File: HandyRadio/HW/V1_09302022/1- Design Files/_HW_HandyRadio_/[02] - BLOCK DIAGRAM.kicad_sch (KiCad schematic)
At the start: 0 parts

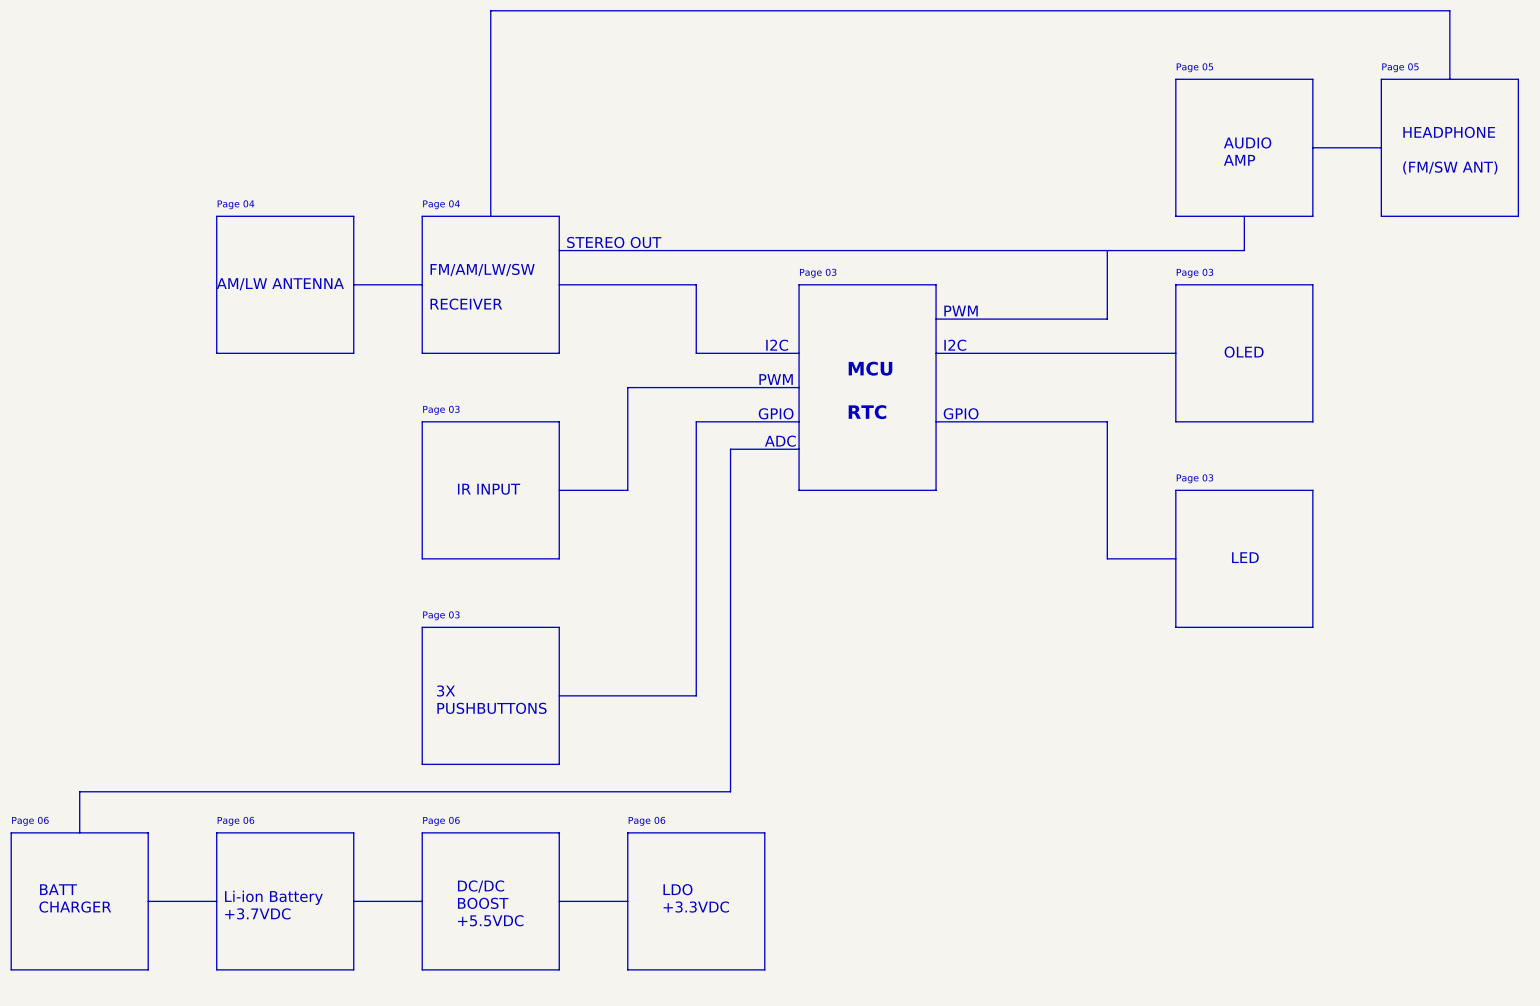
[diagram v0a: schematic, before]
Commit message: almost ready for routing and finishing PCB :D
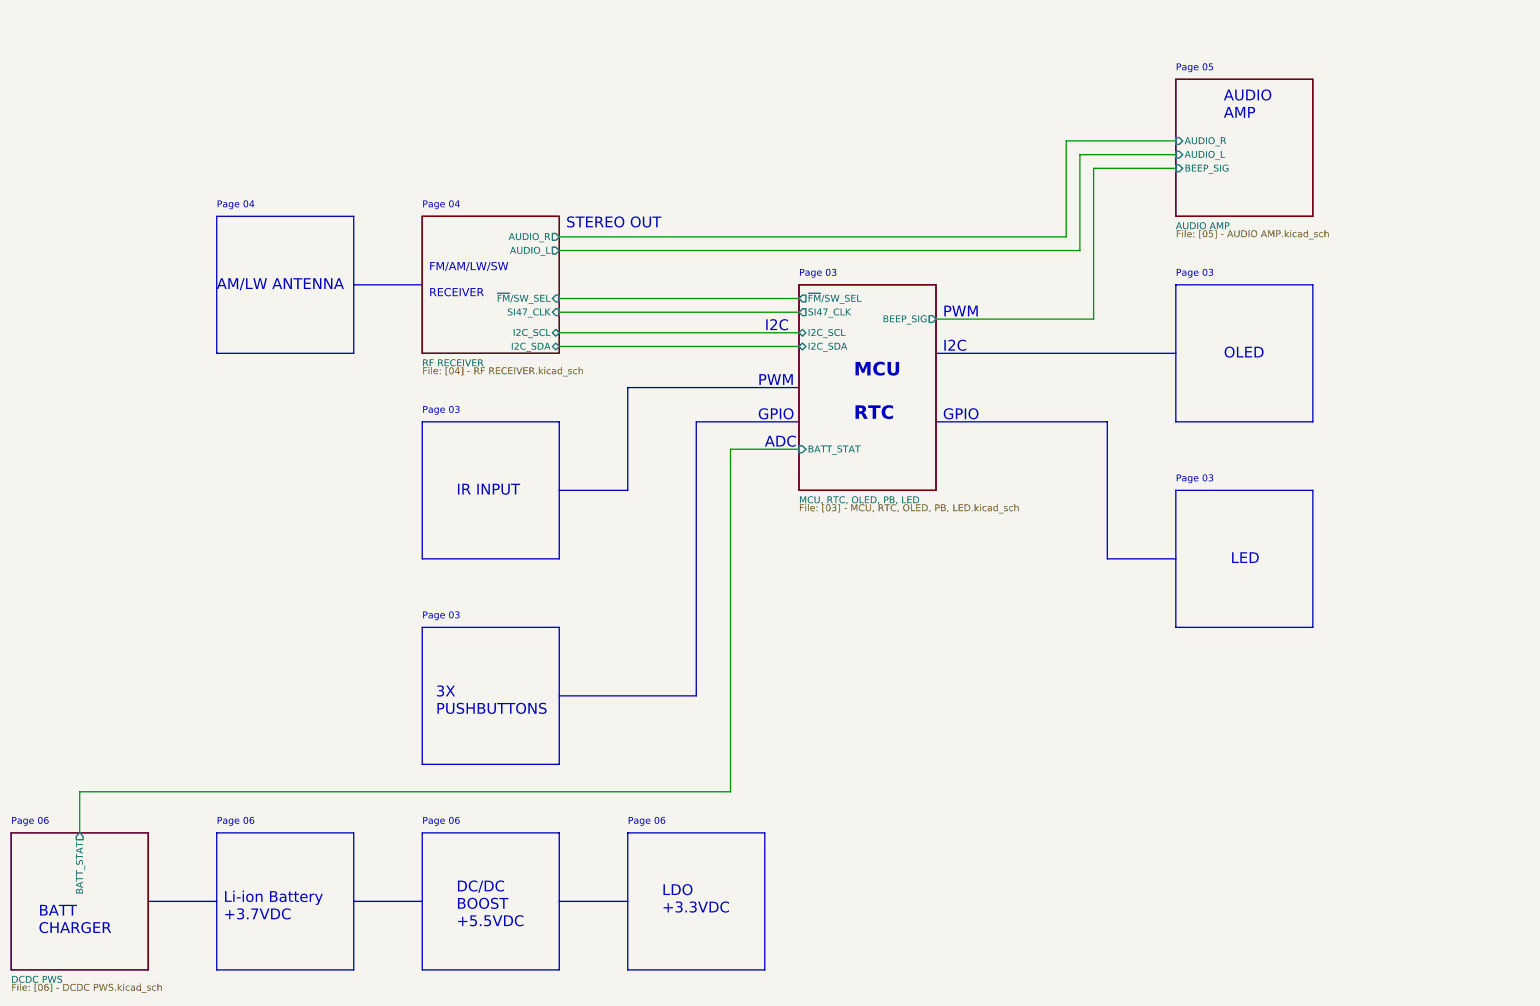
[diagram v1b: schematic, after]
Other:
- added sheet AUDIO AMP ([05] - AUDIO AMP.kicad_sch)
- added sheet DCDC PWS ([06] - DCDC PWS.kicad_sch)
- added sheet MCU, RTC, OLED, PB, LED ([03] - MCU, RTC, OLED, PB, LED.kicad_sch)
- added sheet RF RECEIVER ([04] - RF RECEIVER.kicad_sch)
- note removed: "HEADPHONE (FM/SW ANT)"
